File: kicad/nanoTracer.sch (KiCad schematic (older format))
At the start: 51 parts, among them J1 ARDUINO_UNO_REV3_PINS, P1 6.3_AC, P2 HEATER, P3 CONN_3, P4 HT_AC, P5 NEG_AC, U1 TL072, U2 TL071, U3 MCP4921-E/P, U4 LM337T, U5 MCP3202, U6 SIL12

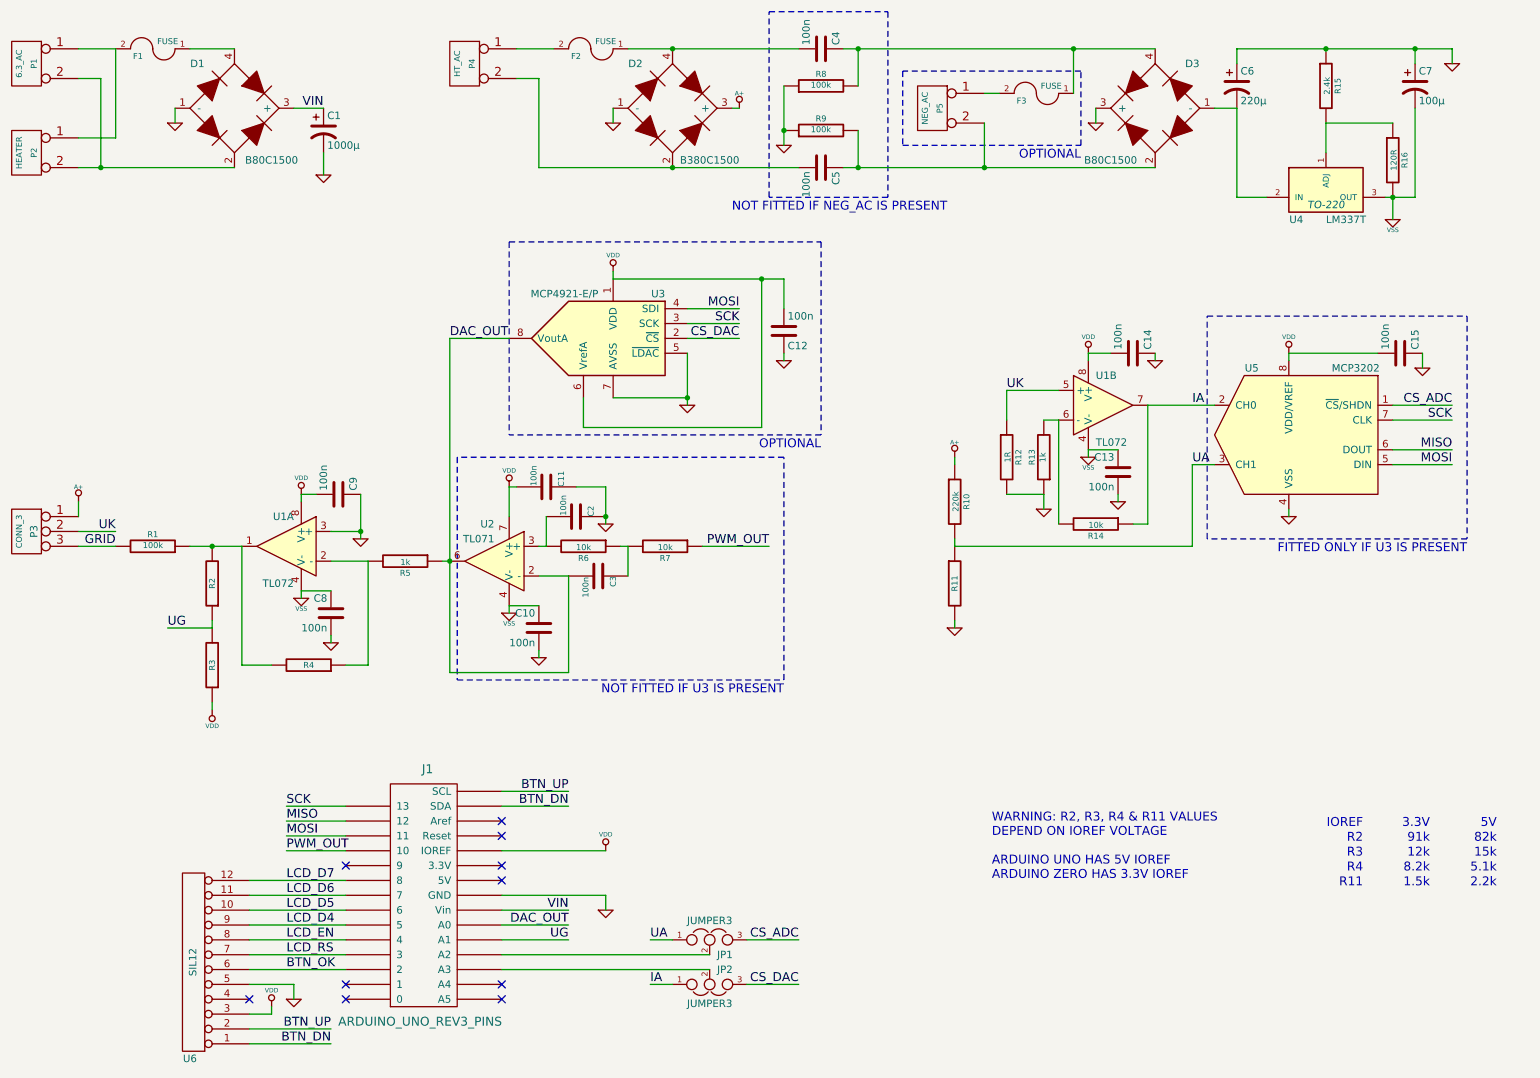
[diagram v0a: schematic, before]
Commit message: Complete footprints association
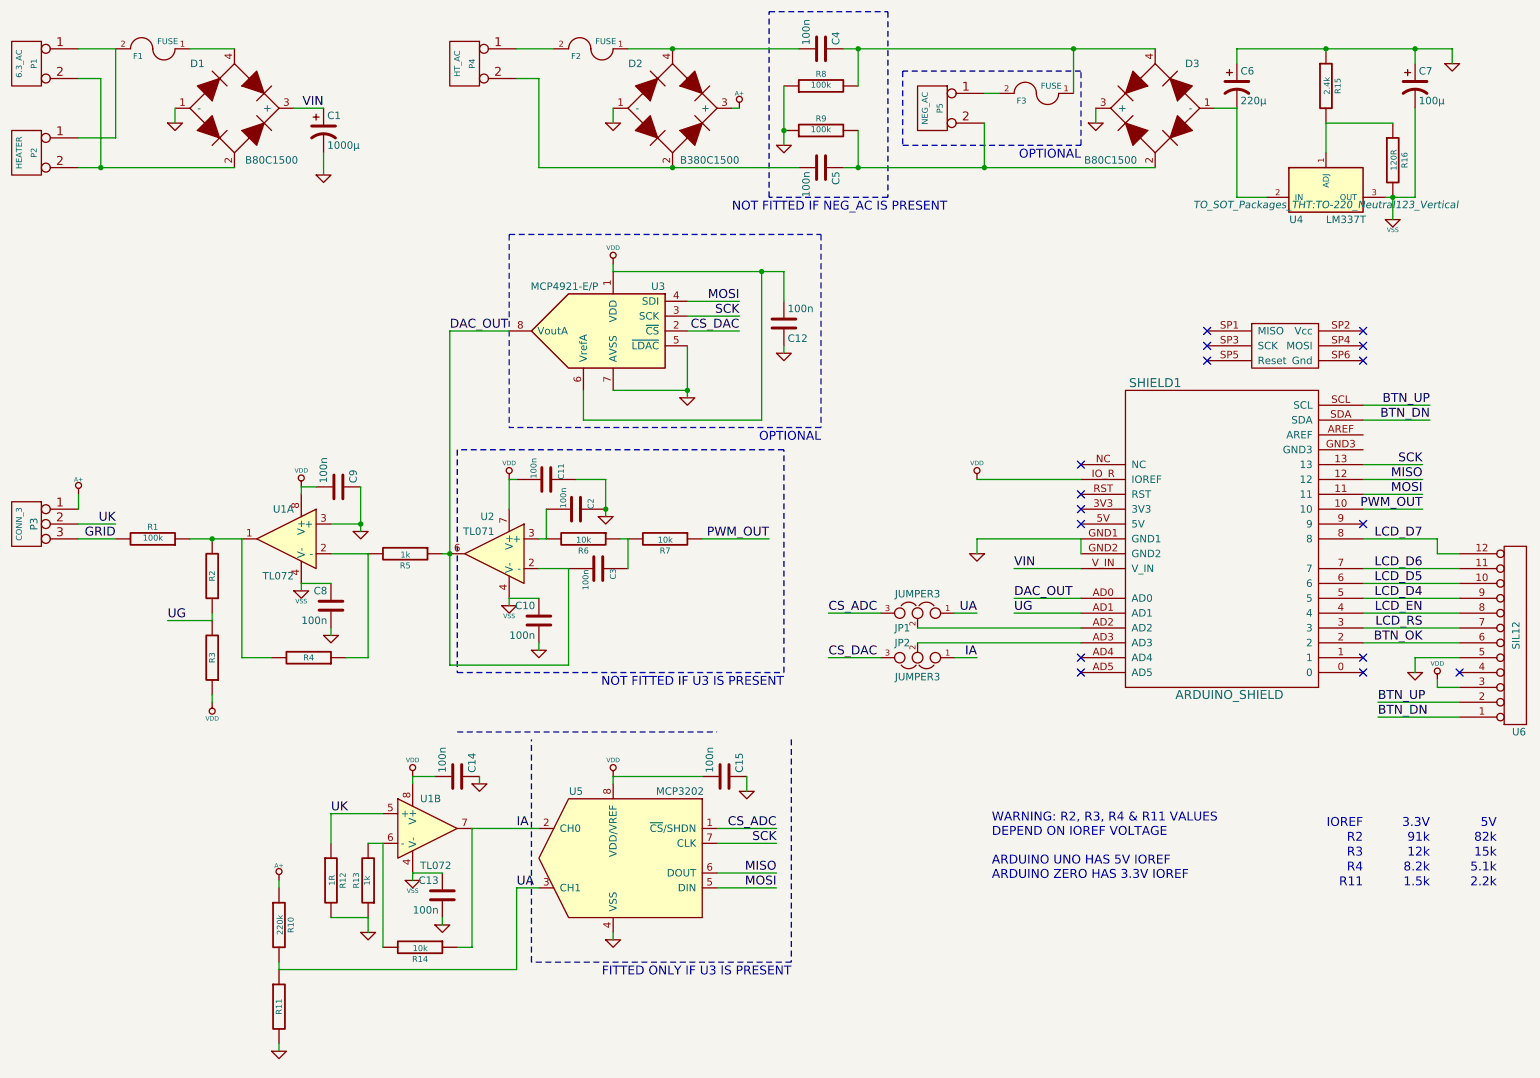
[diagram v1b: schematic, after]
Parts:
- removed J1: ARDUINO_UNO_REV3_PINS, symbol ARDUINO_UNO_REV3_PINS
- added SHIELD1: ARDUINO_SHIELD, freetronics_footprints:ARDUINO_SHIELD, symbol ARDUINO_SHIELD
- C1: footprint (none) -> Capacitors_ThroughHole:C_Radial_D10_L16_P5
- C10, C12, C13, C14, C15, C4, C5, C8, C9: footprint (none) -> Capacitors_ThroughHole:C_Rect_L7_W2_P5
- C11, C2, C3: footprint ~ -> Capacitors_ThroughHole:C_Rect_L7_W2_P5
- C6: footprint (none) -> Capacitors_ThroughHole:C_Radial_D7.5_L11.2_P2.5
- C7: footprint (none) -> Capacitors_ThroughHole:C_Radial_D6.3_L11.2_P2.5
- D1, D2, D3: footprint (none) -> w_pth_diodes:bridge_wob
- F1, F2, F3: footprint ~ -> Fuse_Holders_and_Fuses:Fuseholder5x20_horiz_open_Schurter_0031_8201
- JP1, JP2: footprint (none) -> Pin_Headers:Pin_Header_Straight_1x03
- P1, P2, P4, P5: footprint (none) -> Connect:bornier2
- P3: footprint (none) -> Connect:bornier3
- R1, R10, R11, R12, R13, R14, R15, R16, R2, R3, R4, R5, R6, R7, R8, R9: footprint ~ -> Resistors_ThroughHole:Resistor_Horizontal_RM10mm
- U1, U2, U3, U5: footprint (none) -> Housings_DIP:DIP-8_W7.62mm_LongPads
- U4: footprint TO-220 -> TO_SOT_Packages_THT:TO-220_Neutral123_Vertical
- U6: footprint (none) -> Pin_Headers:Pin_Header_Straight_1x12
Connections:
- net BTN_DN: now also SHIELD1.SDA
- net BTN_OK: now also SHIELD1.2
- net BTN_UP: now also SHIELD1.SCL
- net DAC_OUT: now also SHIELD1.AD0
- net GND: now also SHIELD1.GND1, SHIELD1.GND2
- net LCD_D4: now also SHIELD1.5
- net LCD_D5: now also SHIELD1.6
- net LCD_D6: now also SHIELD1.7
- net LCD_D7: now also SHIELD1.8
- net LCD_EN: now also SHIELD1.4
- net LCD_RS: now also SHIELD1.3
- net MISO: now also SHIELD1.12
- net MOSI: now also SHIELD1.11
- net PWM_OUT: now also SHIELD1.10
- net SCK: now also SHIELD1.13
- net UG: now also SHIELD1.AD1
- net VDD: now also SHIELD1.IO_R (IOREF)
- net VIN: now also SHIELD1.V_IN
- net at JP1.2: now also SHIELD1.AD2
- net at JP2.2: now also SHIELD1.AD3
- no-connect marks 10 -> 16
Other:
- moved on the sheet: C10, C11, C12, C13, C14, C15, C2, C3, C8, C9, JP1, JP2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
